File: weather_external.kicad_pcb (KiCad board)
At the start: 2 copper layers, 15 parts, among them J2 Conn_01x02_Male, SW1 SW_Push

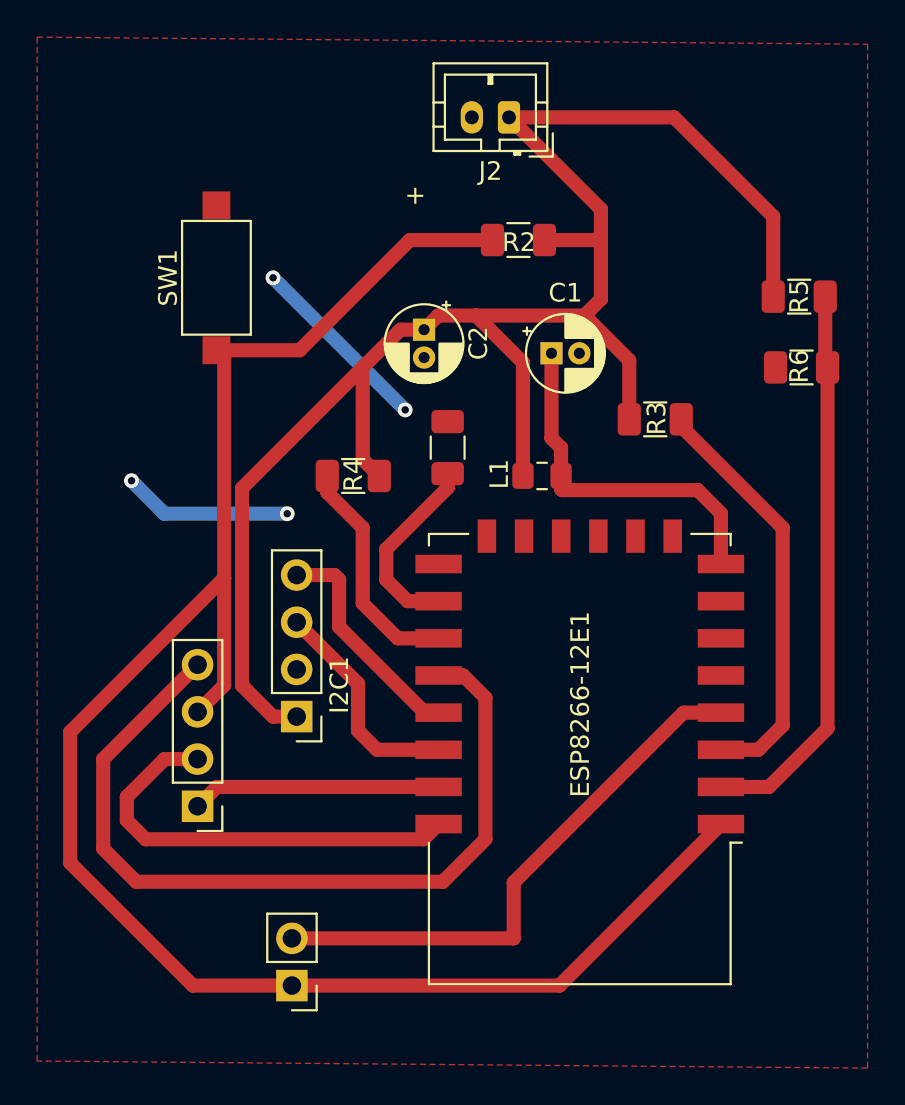
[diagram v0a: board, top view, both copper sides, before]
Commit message: no 555 Print version
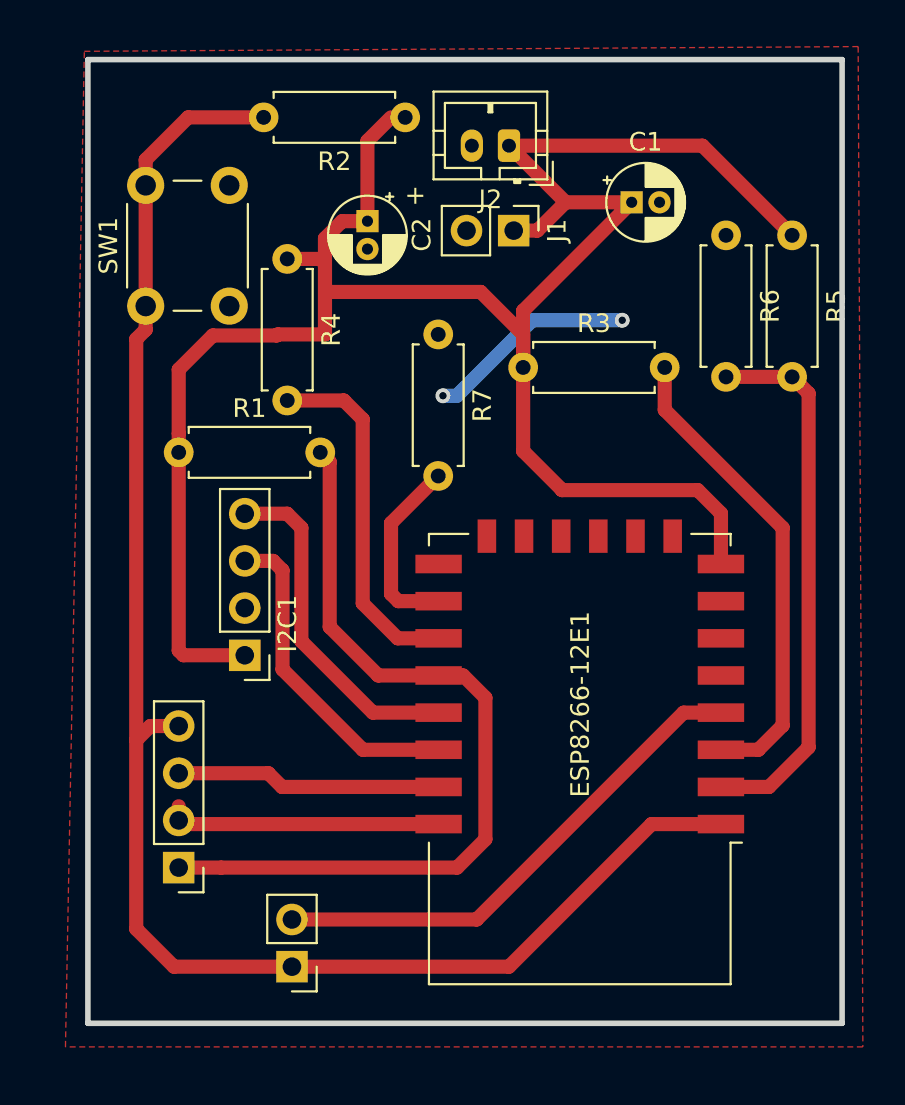
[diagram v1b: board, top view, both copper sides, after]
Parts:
- removed L1: INDUCTOR, Inductor_SMD:L_0805_2012Metric_Pad1.15x1.40mm_HandSolder
- added J1: Conn_01x02_Male, Connector_PinHeader_2.54mm:PinHeader_1x02_P2.54mm_Vertical, F.Cu at (10.9, 60.7)
- added R1: 5k, Resistor_THT:R_Axial_DIN0207_L6.3mm_D2.5mm_P7.62mm_Horizontal, F.Cu at (-7.11, 72.6)
- R2, R3, R4, R5, R6, R7: footprint Resistor_SMD:R_1206_3216Metric -> Resistor_THT:R_Axial_DIN0207_L6.3mm_D2.5mm_P7.62mm_Horizontal
- SW1: footprint Button_Switch_SMD:SW_SPST_CK_RS282G05A3 -> Button_Switch_THT:SW_PUSH_6mm
- moved R4 12.2 mm to (-1.27, 62.2), turned to 270 degrees
- moved C1 9.20 mm to (17.3, 59.2)
- moved R2 8.99 mm to (5.08, 54.6)
- moved R6 8.19 mm to (22.4, 61.0), turned to 270 degrees
- moved R3 7.64 mm to (11.4, 68.1)
- moved C2 6.59 mm to (3.05, 60.2)
- moved R7 6.12 mm to (6.86, 66.3)
- moved I2C1 4.33 mm to (-3.56, 83.6)
- moved SW1 4.10 mm to (-8.89, 64.8)
- moved FTDI1 3.45 mm to (-7.11, 95.0)
- moved R5 3.32 mm to (25.9, 61.0), turned to 270 degrees
- moved J2 1.52 mm to (10.7, 56.1)
- moved JP1 1.02 mm to (-1.02, 100.3)
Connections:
- C1 pad 1: Net-(C1-Pad1) -> +3V3
- ESP8266-12E1 pad 8: Net-(C1-Pad1) -> +3V3
- FTDI1 pad 1: Net-(ESP8266-12E1-Pad21) -> Net-(ESP8266-12E1-Pad18)
- FTDI1 pad 3: Net-(ESP8266-12E1-Pad1) -> Net-(ESP8266-12E1-Pad21)
- FTDI1 pad 4: Net-(ESP8266-12E1-Pad18) -> Net-(ESP8266-12E1-Pad1)
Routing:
- net +3V3: track 96.0 -> 116.1 mm
- net Net-(C1-Pad1): track 19.4 -> 0.00 mm
- net Net-(ESP8266-12E1-Pad1): track 97.9 -> 86.4 mm
- net Net-(ESP8266-12E1-Pad22): track 23.5 -> 15.1 mm
- net GND: track 19.2 -> 11.3 mm, vias 4 -> 2
- net Net-(ESP8266-12E1-Pad19): track 12.2 -> 19.2 mm
- net Net-(ESP8266-12E1-Pad17): track 12.5 -> 19.3 mm
- net Net-(ESP8266-12E1-Pad20): track 12.0 -> 17.8 mm
- net Net-(ESP8266-12E1-Pad3): track 22.6 -> 25.8 mm
- net Net-(ESP8266-12E1-Pad4): track 29.9 -> 27.7 mm
- net Net-(ESP8266-12E1-Pad21): track 13.4 -> 14.3 mm
- net Net-(ESP8266-12E1-Pad2): track 30.3 -> 29.5 mm
- net Net-(ESP8266-12E1-Pad18): track 44.9 -> 44.3 mm
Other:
- board outline added: 40.6 x 51.9 mm
